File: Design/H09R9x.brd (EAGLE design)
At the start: 34.6 x 30 mm, 25 parts, among them P1 HEXABIT_17.32, U2 TSD305-1C55, X1 XTALL_CSTCE8M00G52

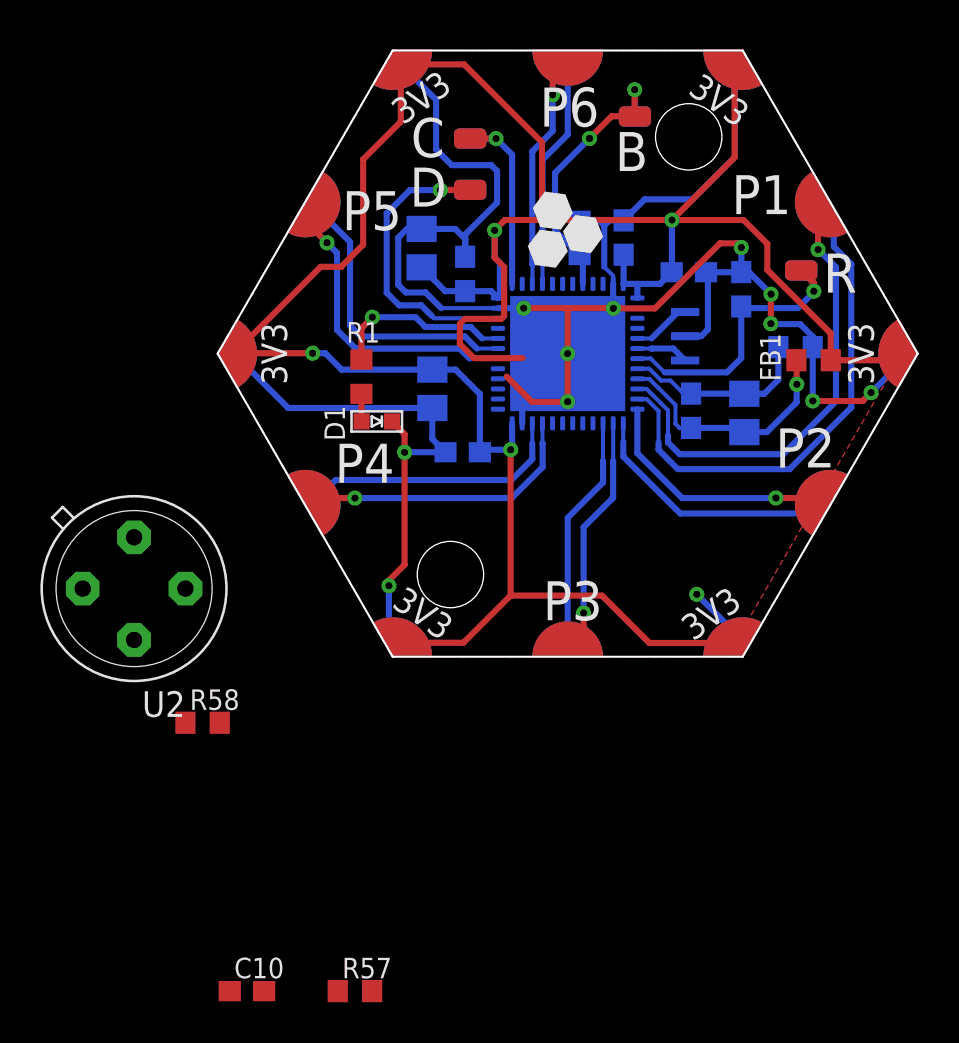
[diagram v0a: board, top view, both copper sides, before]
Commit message: first version sch brd .
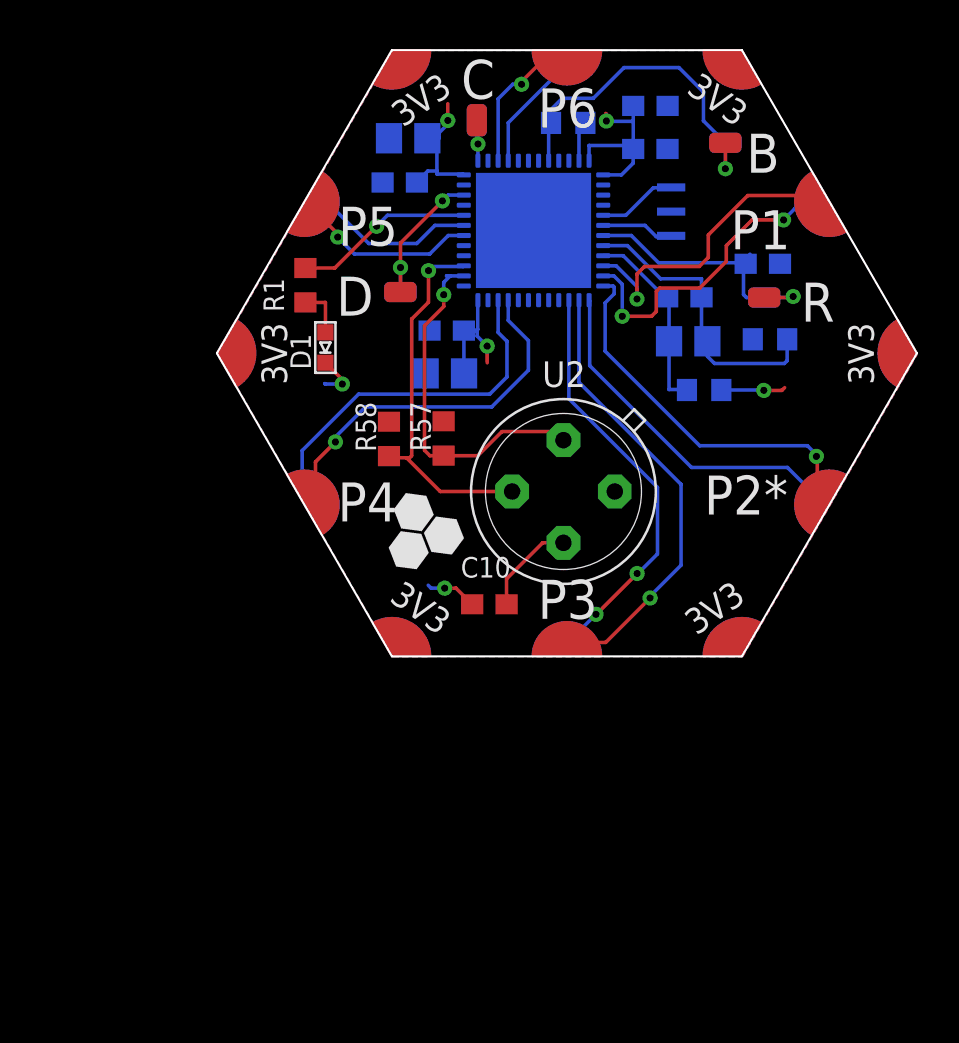
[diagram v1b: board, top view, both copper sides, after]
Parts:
- C2, C4, C7: device Hexabitz:C-0805-POL -> Hexabitz:C-0805
- moved R57 27.7 mm to (28.5, 30.4), turned to 90 degrees
- moved C10 22.6 mm to (30.7, 22.2), turned to 180 degrees
- moved U2 21.8 mm to (34.4, 27.8), turned to 90 degrees
- moved R58 16.8 mm to (25.8, 30.4), turned to 90 degrees
- moved C6 6.65 mm to (38.7, 46.9), turned to 180 degrees
- moved C9 6.39 mm to (38.7, 44.7)
- moved U1 6.33 mm to (32.9, 40.7)
- moved X1 6.20 mm to (39.7, 41.6)
- moved D 6.12 mm to (26.3, 37.7), turned to 0 degrees
- moved C5 6.07 mm to (28.6, 35.8)
- moved R3 5.72 mm to (34.6, 46.0), turned to 0 degrees
- moved C1 5.62 mm to (40.4, 37.4), turned to 180 degrees
- moved FB1 5.61 mm to (41.4, 32.8), flipped to the bottom, turned to 180 degrees
- moved C3 5.56 mm to (26.3, 43.1), turned to 0 degrees
- moved C4 5.48 mm to (26.7, 45.3), turned to 0 degrees
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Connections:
- net SCL renamed I2C2_SCL
- net SDA renamed I2C2_SDA
- net USART2_RX renamed USART2_RX*
- net USART2_TX renamed USART2_TX*
- removed net +3V3: C10.1, R57.2, R58.2, U2.3
- removed net BLED: U1.P$19
- removed net GLED: U1.P$18
- removed net RLED: U1.P$17
- new net INT: U1.P$20
- net GND: now also U1.P$17, U1.P$18, U1.P$45, U1.P$46
- net VDD: now also C10.1, R57.2, R58.2, U2.3
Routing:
- net GND: track 129.8 -> 6.85 mm, vias 12 -> 2
- net VDD: track 135.7 -> 30.6 mm
- net I2C2_SDA: track 0.00 -> 18.6 mm, vias 0 -> 1
- net I2C2_SCL: track 0.00 -> 17.7 mm, vias 0 -> 1
- net USART6_TX: track 11.8 -> 22.5 mm
- net USART4_RX: track 24.9 -> 15.6 mm, vias 0 -> 2
- net USART6_RX: track 11.6 -> 20.7 mm, vias 0 -> 2
- net N$7: track 16.1 -> 7.77 mm, vias 1 -> 2
- net USART4_TX: track 23.2 -> 15.4 mm
- net N$9: track 10.1 -> 3.31 mm
- net USART2_TX*: track 12.0 -> 18.7 mm
- net USART1_TX: track 15.0 -> 8.80 mm
- net USART1_RX: track 14.2 -> 8.37 mm
- net USART5_RX: track 11.4 -> 5.99 mm
- net VSSA: track 9.39 -> 14.7 mm
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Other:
- board text added: "H08R60"
- board text added: "P2*"
- board text removed: "H01R01"
- board text removed: "P2"
